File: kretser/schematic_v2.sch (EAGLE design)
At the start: 16 parts, among them IC1 ATMEGA168-20PU, U2 LM2940CT-5.0/NOPB

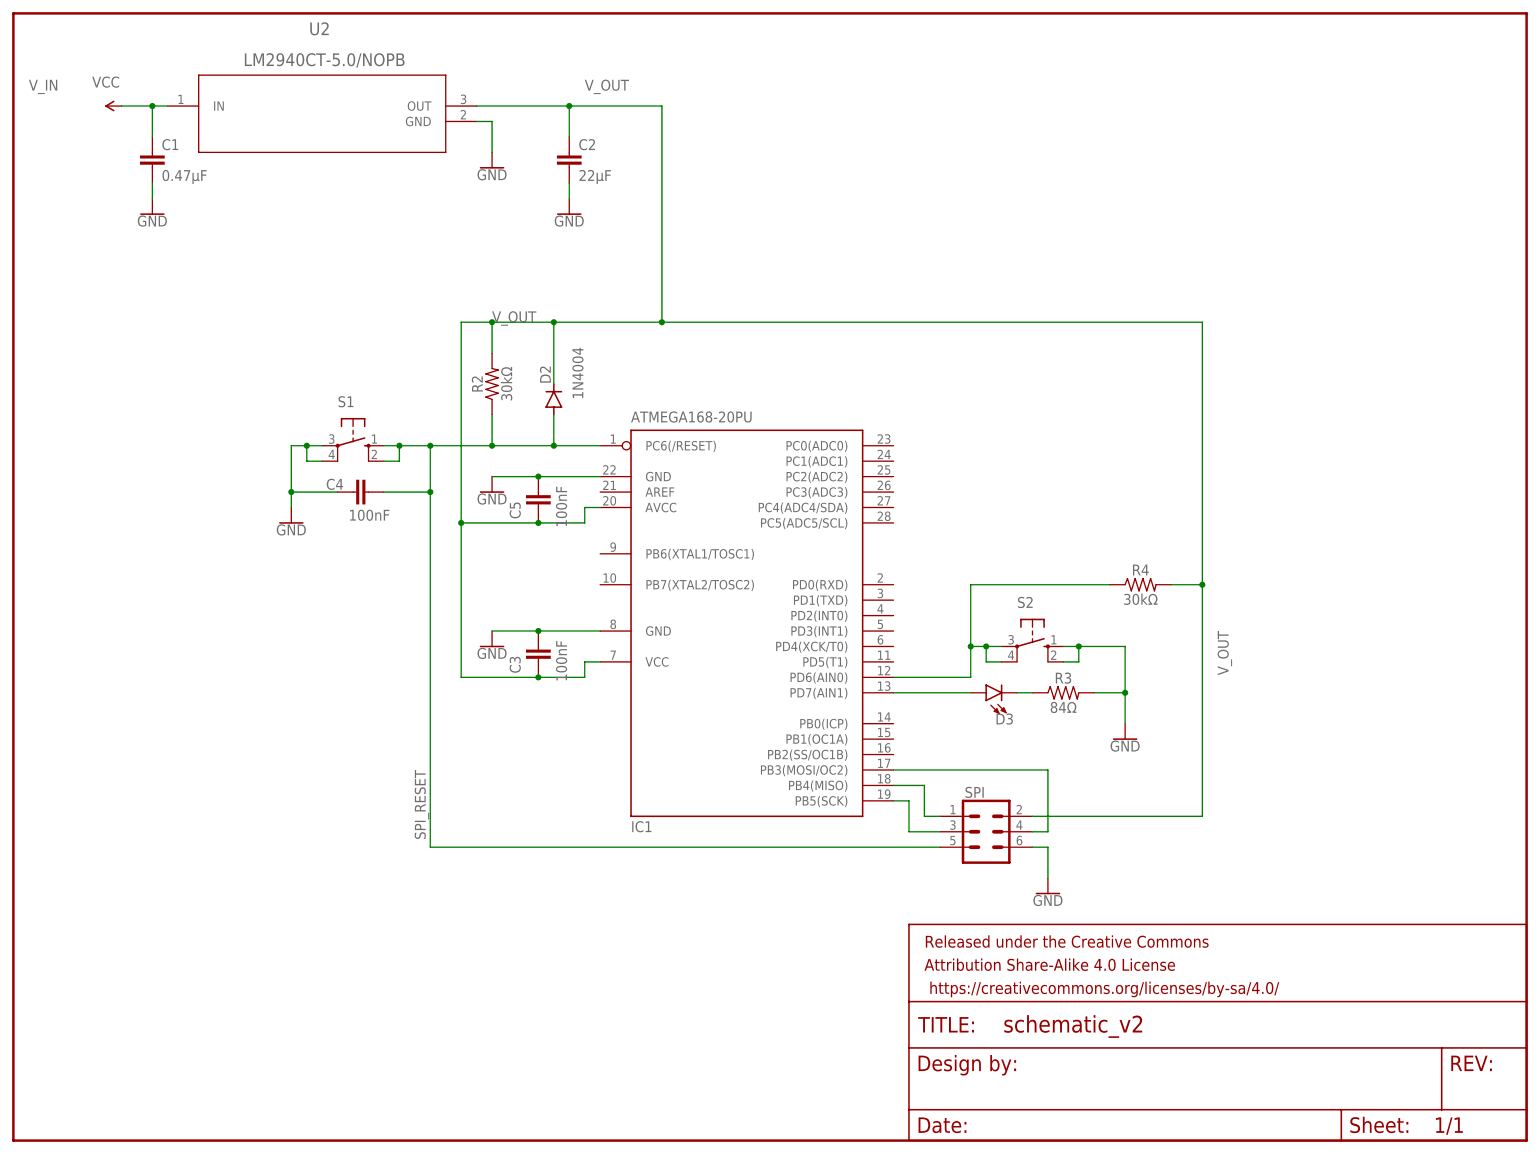
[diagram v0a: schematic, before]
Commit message: updated krets, updated programs
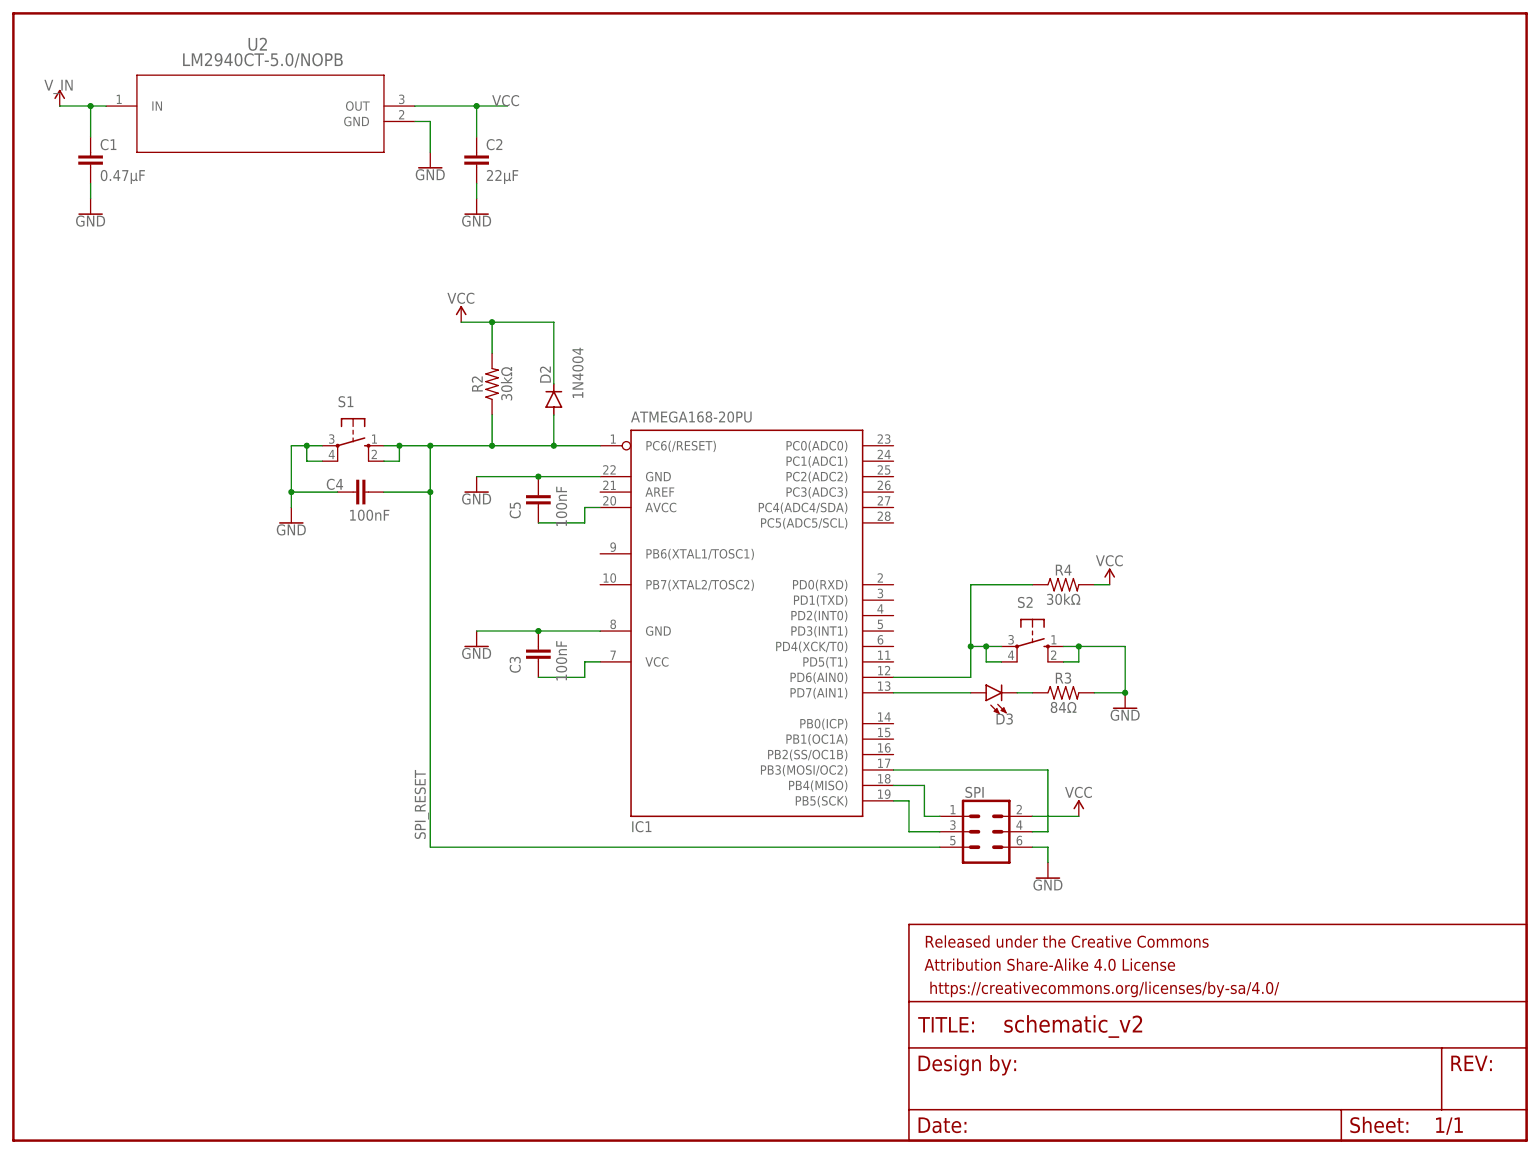
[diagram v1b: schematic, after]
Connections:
- removed net V_OUT: C2.1, C3.1, C5.1, D2.C, IC1.AVCC, IC1.VCC@1, R2.2, R4.2, SPI.2, U2.OUT
- new net N$2: C3.1, IC1.VCC@1
- new net N$5: C5.1, IC1.AVCC
- new net VCC: C2.1, D2.C, R2.2, R4.2, SPI.2, U2.OUT
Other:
- note added: "LDO_MODULE"
- moved on the sheet: C1, C2, R4, U2
